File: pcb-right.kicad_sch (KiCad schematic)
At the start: 38 parts, among them SW19 GENERIC_ELECTROMECHANICAL_PUS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, SW20 GENERIC_ELECTROMECHANICAL_PUS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, SW21 GENERIC_ELECTROMECHANICAL_PUS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, SW22 GENERIC_ELECTROMECHANICAL_PUS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, SW23 GENERIC_ELECTROMECHANICAL_PUS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, SW24 GENERIC_ELECTROMECHANICAL_PUS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, SW25 GENERIC_ELECTROMECHANICAL_PUS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, SW26 GENERIC_ELECTROMECHANICAL_PUS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, SW27 GENERIC_ELECTROMECHANICAL_PUS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, SW28 GENERIC_ELECTROMECHANICAL_PUS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, SW29 GENERIC_ELECTROMECHANICAL_PUS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, SW30 GENERIC_ELECTROMECHANICAL_PUS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, SW31 GENERIC_ELECTROMECHANICAL_PUS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, SW32 GENERIC_ELECTROMECHANICAL_PUS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, SW33 GENERIC_ELECTROMECHANICAL_PUS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, SW34 GENERIC_ELECTROMECHANICAL_PUS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, SW35 GENERIC_ELECTROMECHANICAL_PUS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, SW36 GENERIC_ELECTROMECHANICAL_PUS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, U2 XIAO-RP2040-DIP

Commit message: Touchups and name: Logos
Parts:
- U2: footprint Seeed Studio XIAO Series Library:XIAO-RP2040-DIP -> benri-projects:SEEED_XIAO-RP2040_T-DIP
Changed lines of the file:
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@@
 			)
 		)
-		(property "Footprint" "Seeed Studio XIAO Series Library:XIAO-RP2040-DIP"
+		(property "Footprint" "benri-projects:SEEED_XIAO-RP2040_T-DIP"
 			(at 226.568 131.318 0)
 			(effects

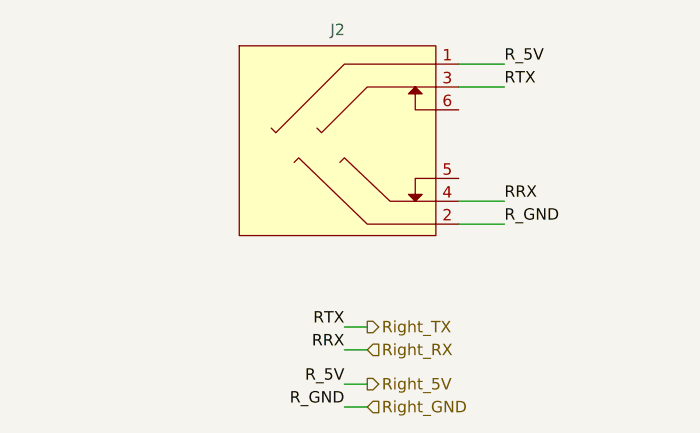
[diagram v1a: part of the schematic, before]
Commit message: Latest release
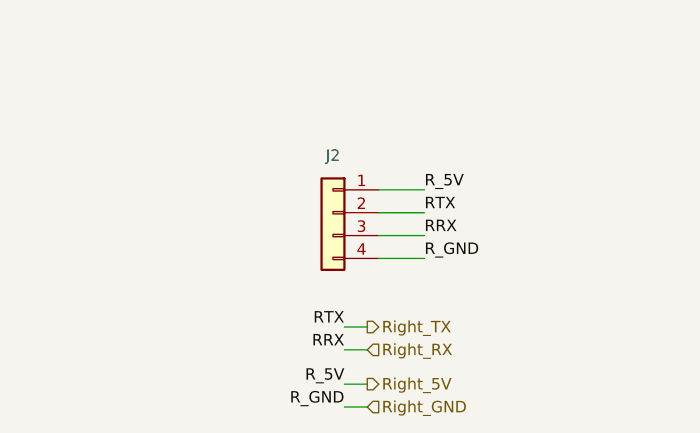
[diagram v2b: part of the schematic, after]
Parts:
- removed J2: ~, benri-projects:TENSILITY_54-00176_R, symbol benri-projects:CONNECTOR_TENSILITY_54-00176
- added J2: (no value), symbol benri-projects:CONNECTOR_JST_SM04B-SRSS-TB
- U2: footprint benri-projects:SEEED_XIAO-RP2040_T-DIP -> Module:MOUDLE14P-XIAO-DIP-SMD
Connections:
- net Right_5V: now also J2.1
- net Right_GND: now also J2.4
- net Right_RX: now also J2.3
- net Right_TX: now also J2.2
